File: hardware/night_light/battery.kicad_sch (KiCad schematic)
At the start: 15 parts, among them J3 JST PH, Q1 AO3401A, U3 MCP73832-2-OT

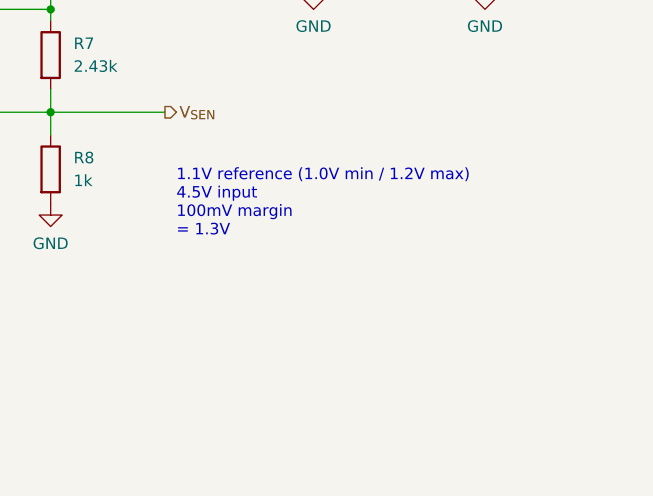
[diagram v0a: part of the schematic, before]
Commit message: working
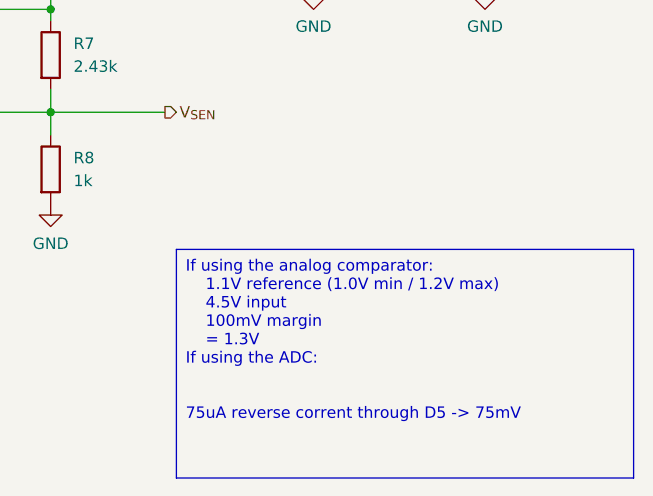
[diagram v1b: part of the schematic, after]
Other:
- note removed: "1.1V reference (1.0V min / 1.2V max) 4.5V input 100mV margin = 1.3V"
